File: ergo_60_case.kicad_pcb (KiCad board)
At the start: 2 copper layers, 285 x 94.6 mm, 166 parts, among them SW1 SW_Push, U1 PRTR5V0U2X, U2 OLED_SSD1306, U3 AT90USB1286-AU, U4 AVR-ISP, Y1 16MHz

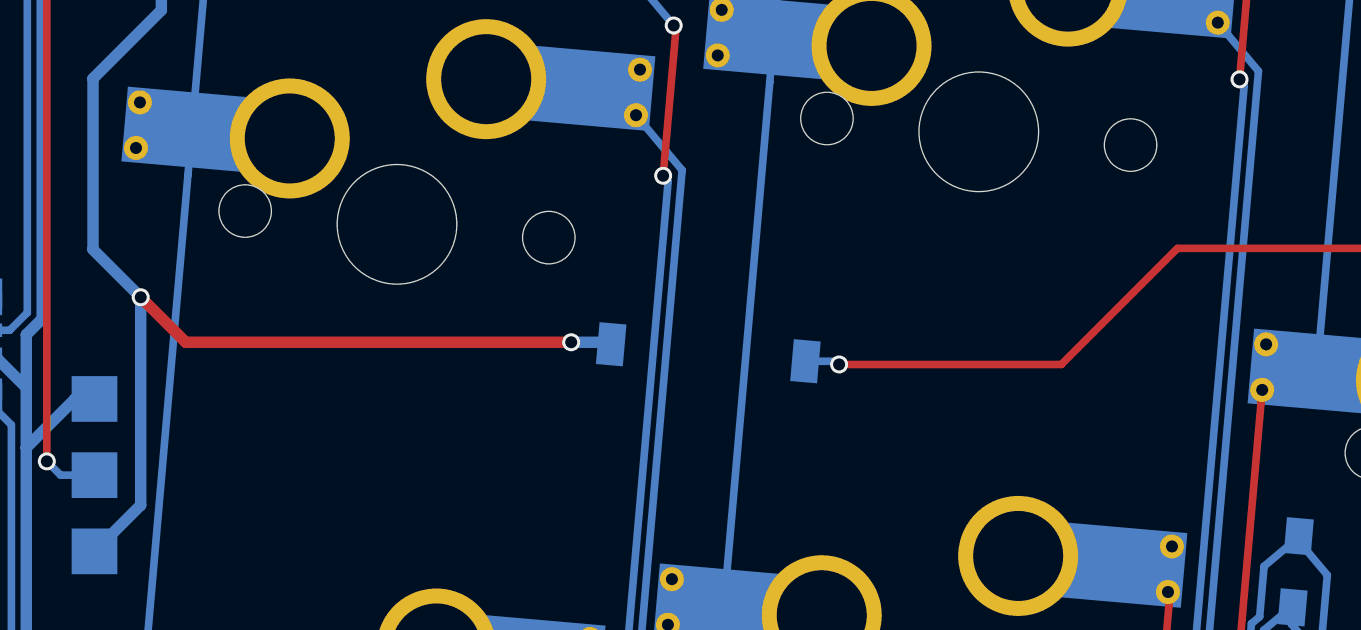
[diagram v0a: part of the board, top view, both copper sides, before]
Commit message: Revert "Revert "reset switch footprint correction""
This reverts commit 81e907175ec75a46385aedb48e9c2c01624081a1.
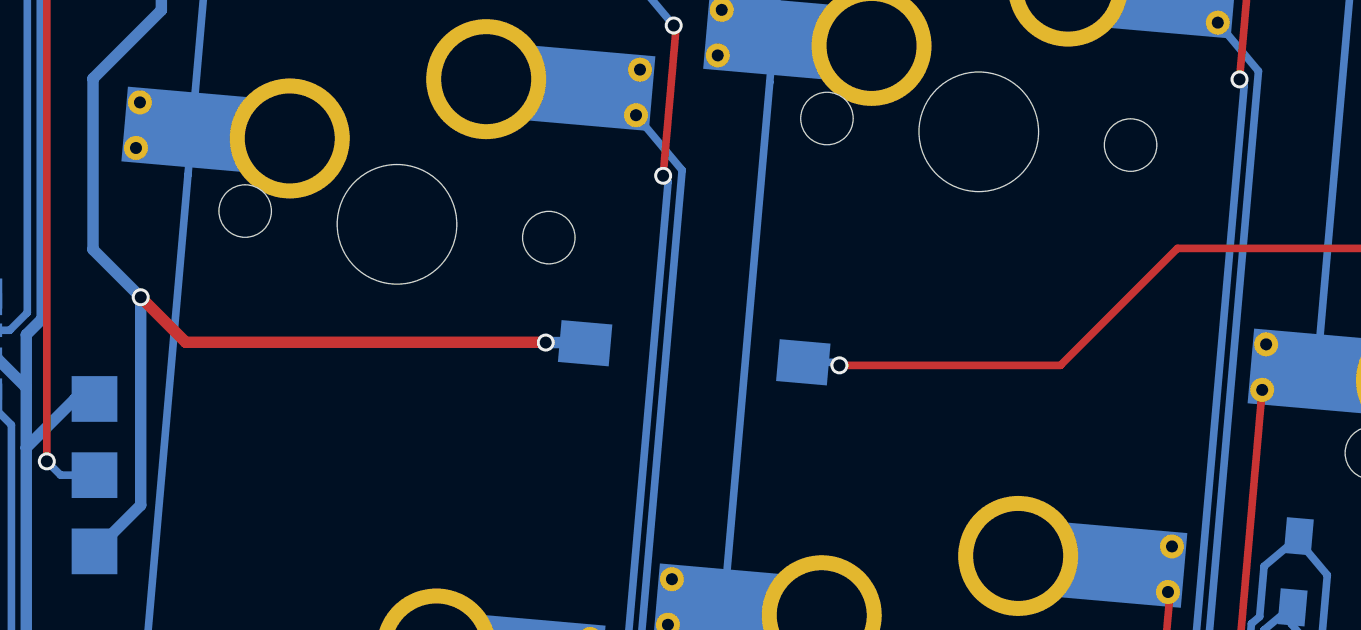
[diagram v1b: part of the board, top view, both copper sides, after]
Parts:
- moved SW1 0.47 mm to (92.8, 124.0)
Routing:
- net GND: track 1335.1 -> 1334.2 mm
